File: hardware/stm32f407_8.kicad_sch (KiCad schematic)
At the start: 28 parts, among them J10 Conn_01x04, J8 GMSB0531112YEU, J9 Conn_01x04, SW3 SW TACT-SPST, U7 STM32F407VGT6, Y3 ABM8G-8.000MHZ-18-D2Y-T

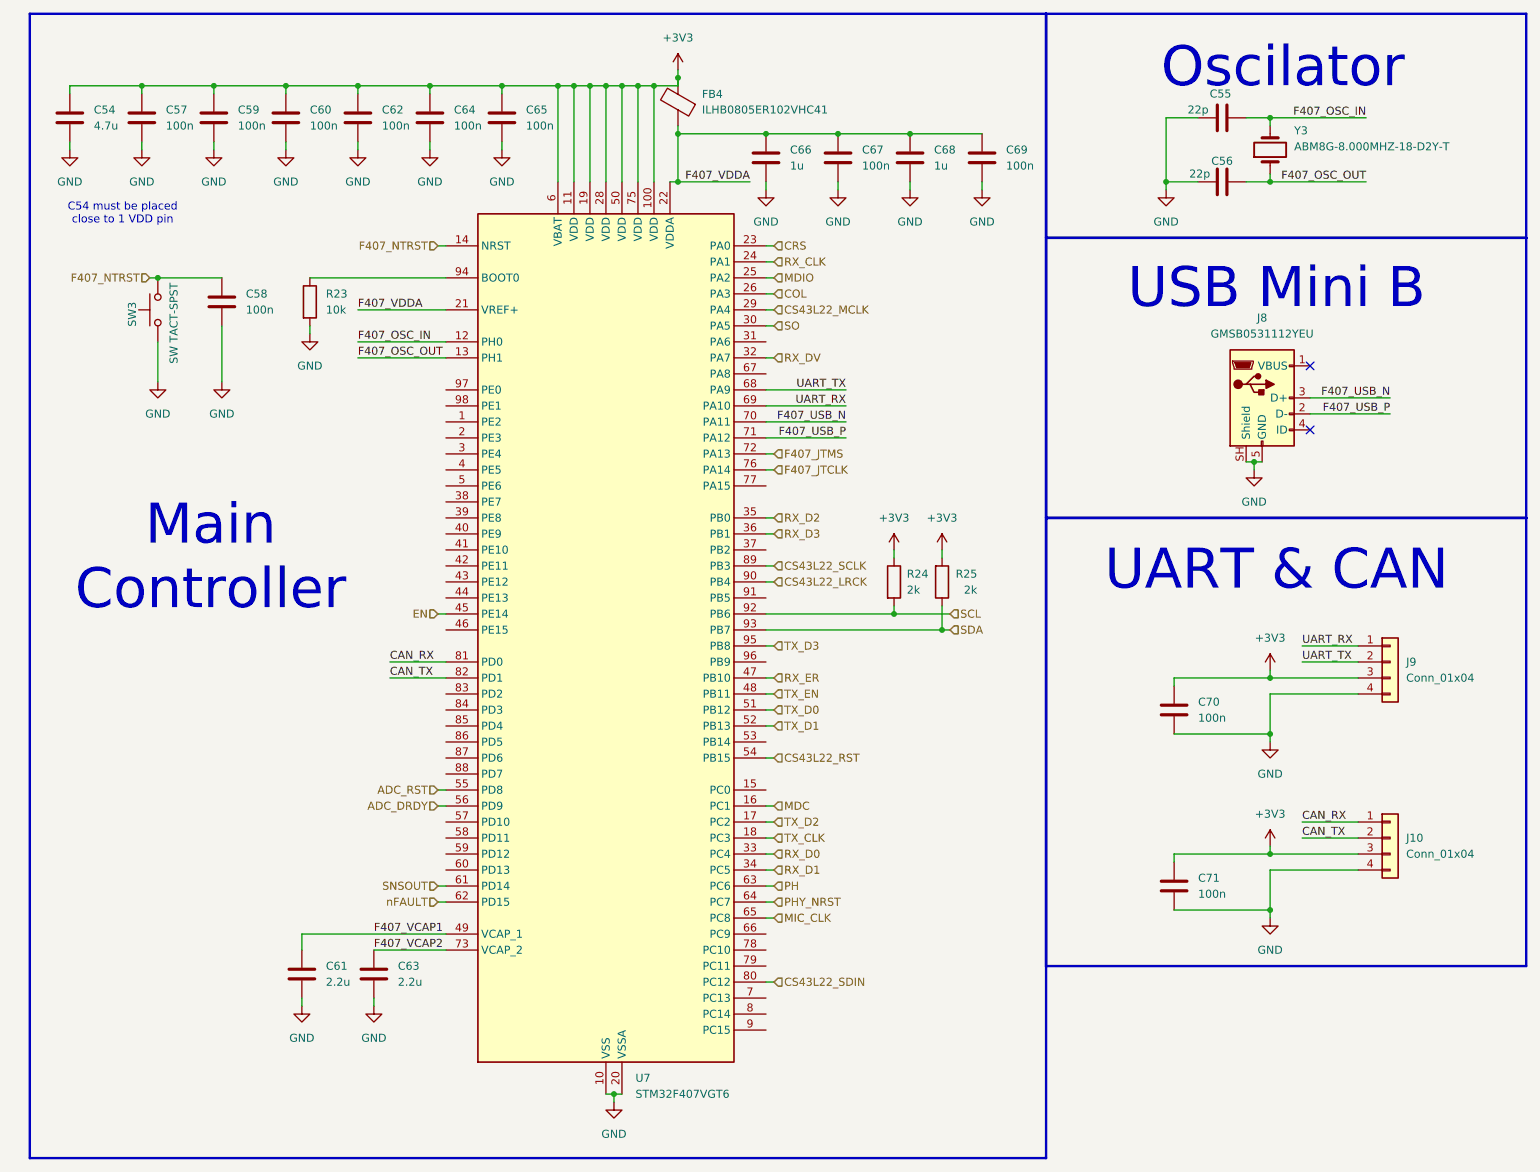
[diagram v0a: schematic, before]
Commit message: Convert Schematic to PCB
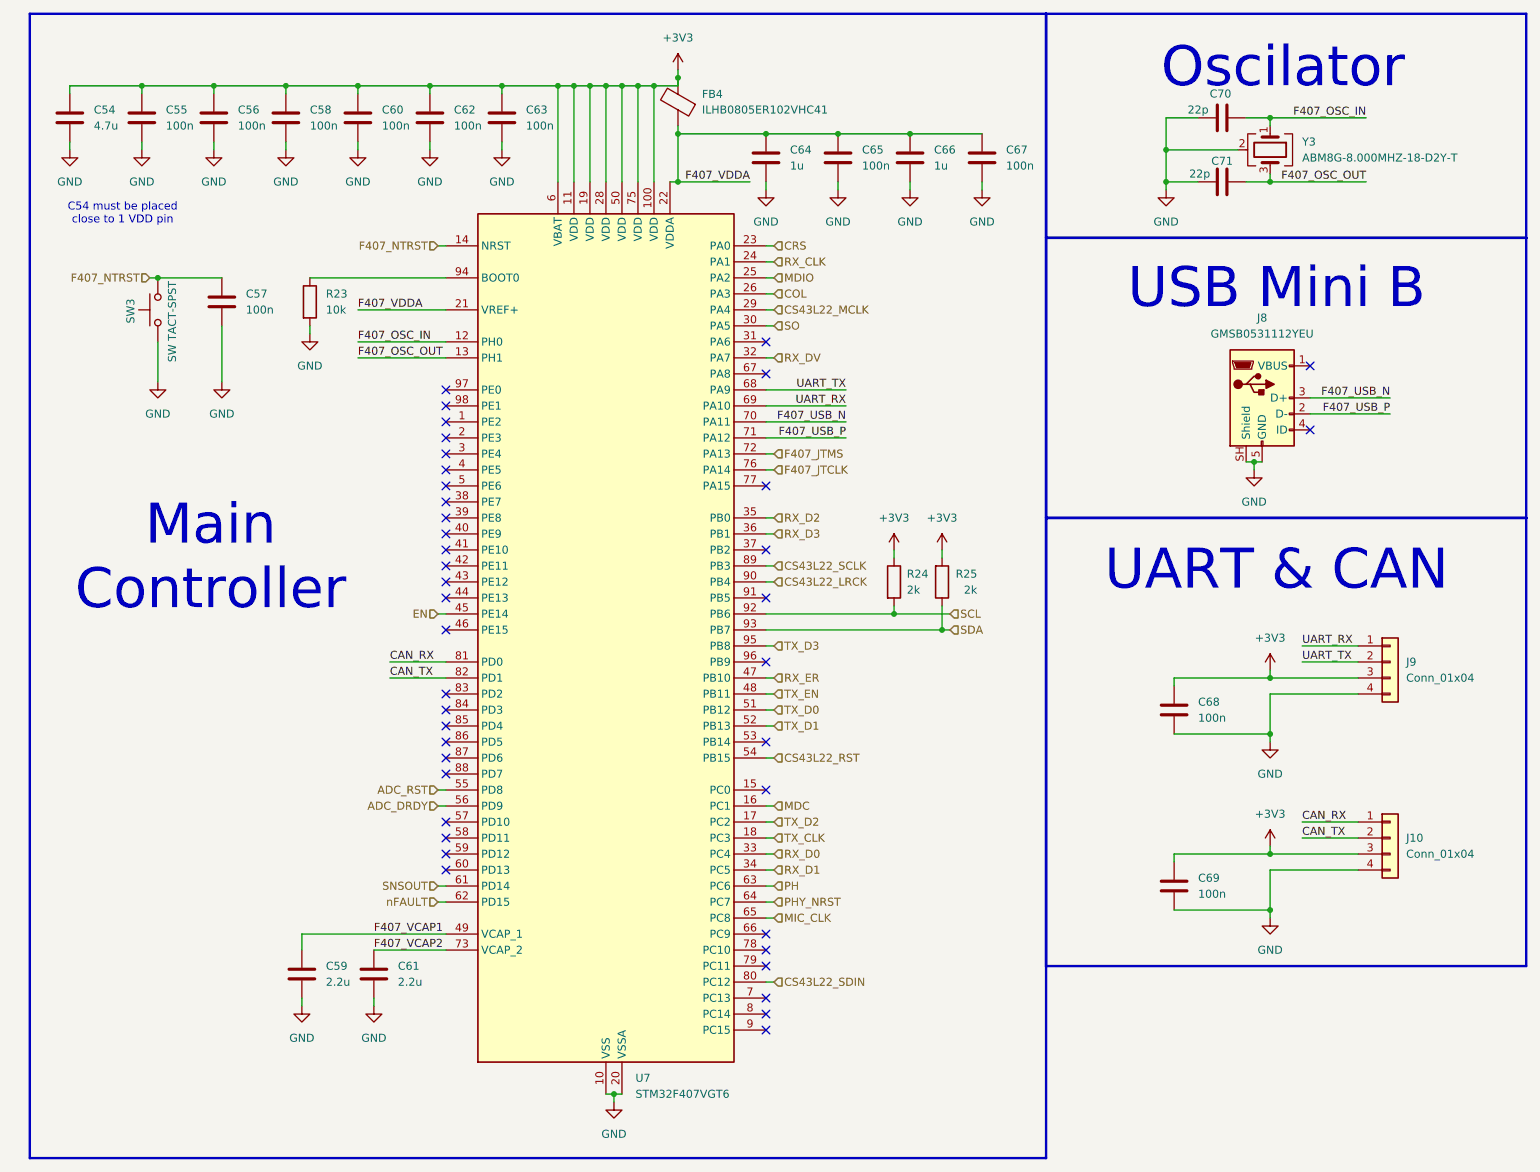
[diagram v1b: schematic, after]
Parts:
- removed SW3: SW TACT-SPST, STM32F407 Dev Kit Library:SW_Push_1P1T_NO_CK_KSC9xxG, symbol Switch:SW_MEC_5G
- removed Y3: ABM8G-8.000MHZ-18-D2Y-T, STM32F407 Dev Kit Library:Crystal_SMD_3225-4Pin_3.2x2.5mm_HandSoldering, symbol Device:Crystal
- added SW3: SW TACT-SPST, STM32F407 Dev Kit Library:SW_Push_SPST_NO_Alps_SKRK, symbol Switch:SW_Push
- added Y3: ABM8G-8.000MHZ-18-D2Y-T, STM32F407 Dev Kit Library:Crystal_SMD_3225-4Pin_3.2x2.5mm_HandSoldering, symbol Device:Crystal_GND24
- renumbered C57 to C55, C59 to C56, C58 to C57, C60 to C58, C61 to C59, C62 to C60, C63 to C61, C64 to C62, C65 to C63, C66 to C64, C67 to C65, C68 to C66, C69 to C67, C70 to C68, C71 to C69, C55 to C70, C56 to C71
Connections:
- net F407_NTRST: now also SW3.2
- net F407_OSC_IN: now also Y3.1
- net F407_OSC_OUT: now also Y3.3
- net GND: now also SW3.1, Y3.2 (G), Y3.4 (G)
- no-connect marks 2 -> 41
